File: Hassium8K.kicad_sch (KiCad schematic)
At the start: 52 parts, among them J1 Conn_01x04_Pin, J2 Conn_01x04_Pin, J3 Conn_01x04_Pin, J4 Conn_01x04_Pin, J5 C596731, J6 C596731, J7 Conn_01x08_Pin, SW1 SW_DPST_x2, SW2 SW_DPST_x2, SW3 SW_DPST_x2, SW4 SW_DPST_x2, U1 STM32H723VGTx, U2 USB3300-EZK, U3 XC6206PxxxMR, U4 STM32F072CBTx, Y1 C5261152, Y2 C9002

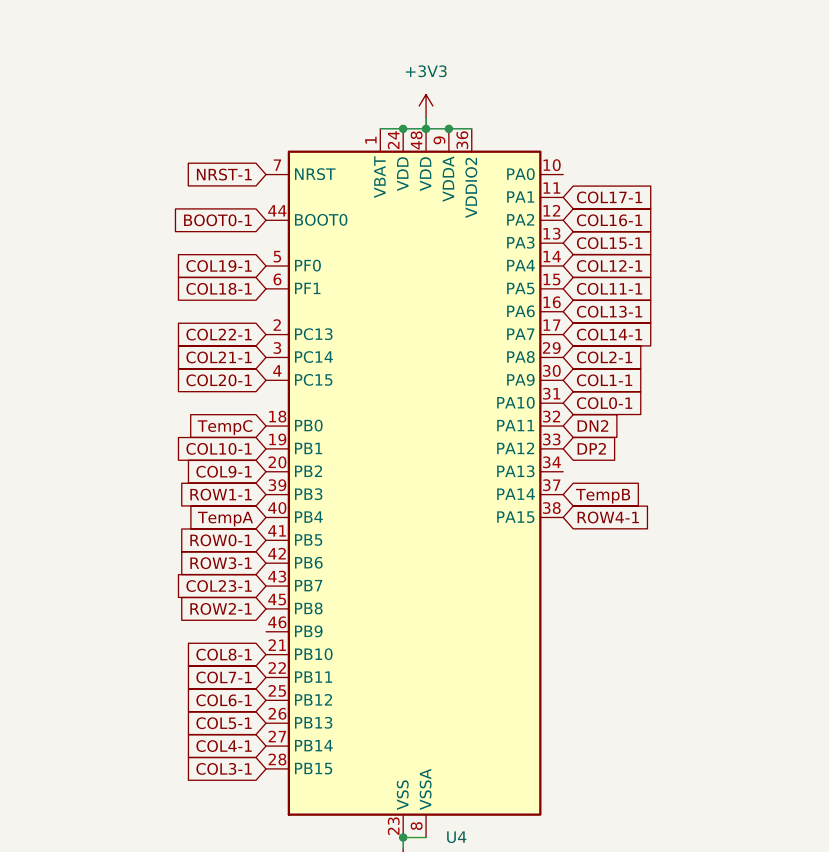
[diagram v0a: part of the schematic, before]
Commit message: Add files via upload
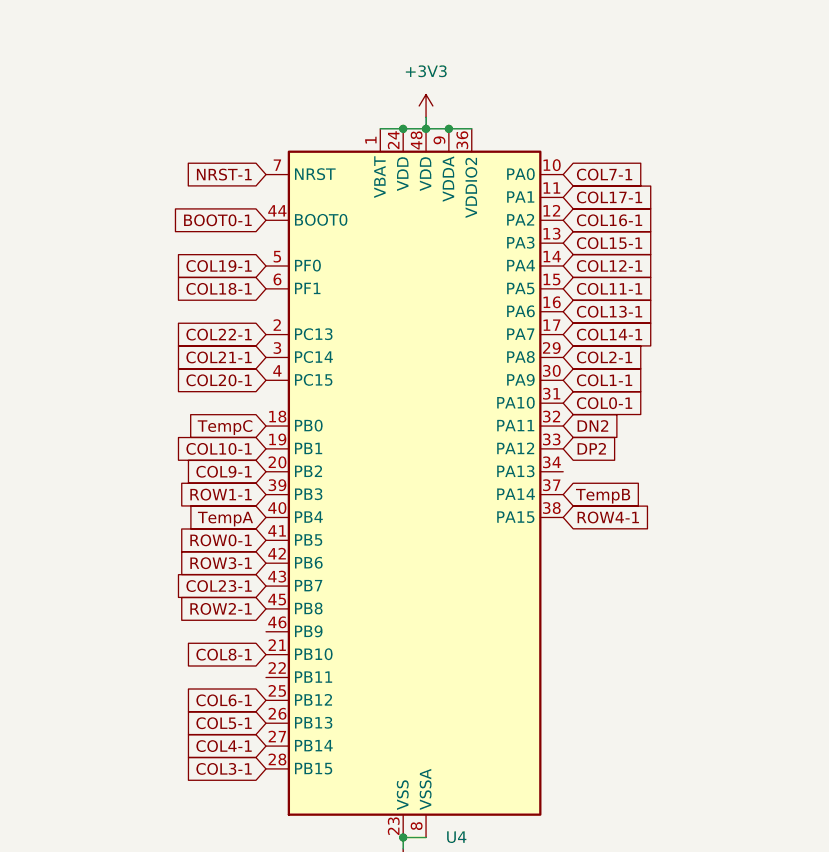
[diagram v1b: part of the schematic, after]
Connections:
- net COL7-1: now also U4.10 (PA0); no longer U4.22 (PB11)
